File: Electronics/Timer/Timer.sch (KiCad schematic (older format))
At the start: 21 parts, among them J1 RJ12-UNSHLD, U1 74HC165, U2 MIC5504-3.3YM5

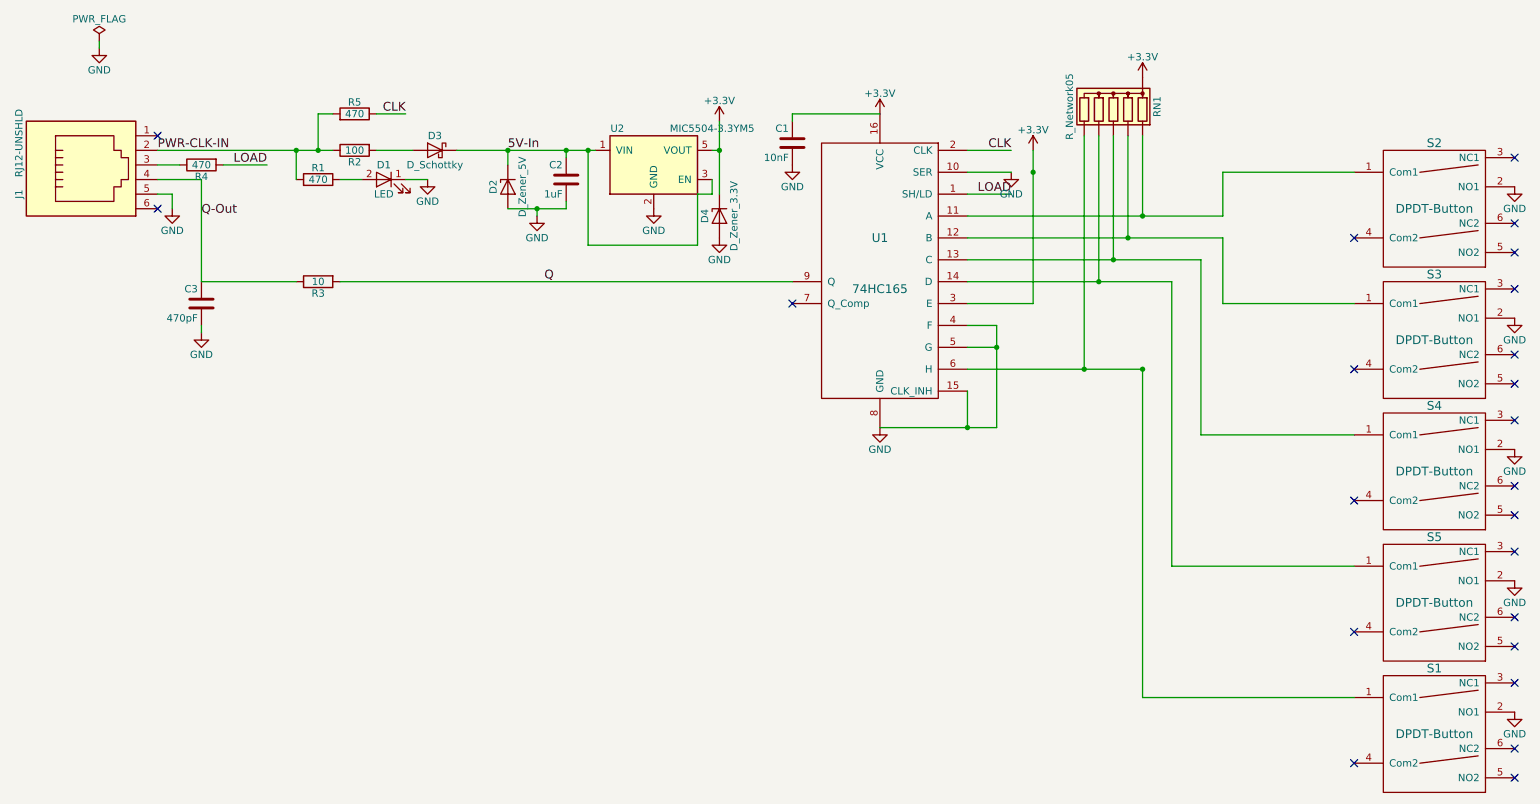
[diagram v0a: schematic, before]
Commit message: Revert "Merge branch 'master' into electronics-tweaks; overwrite 'master' hat changes"
This reverts commit 8490e2c3782f3b2eaf596155d8884dc6cd65858c, reversing
changes made to 143268d8e254d2edd056497eb53e137ee58f0f7c.
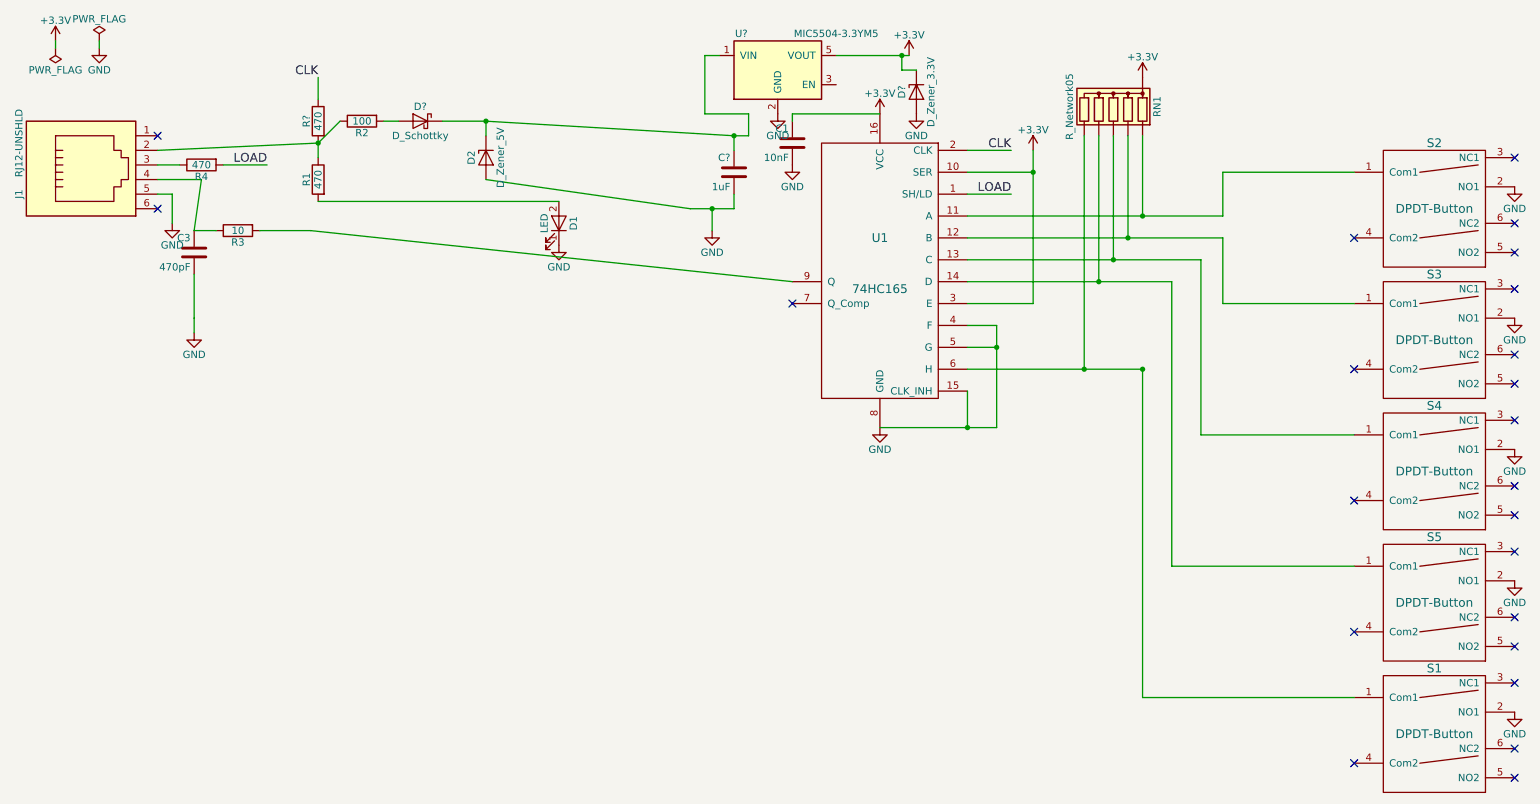
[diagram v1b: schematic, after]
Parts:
- C1: footprint Capacitors_SMD:C_0805_HandSoldering -> Capacitors_SMD:C_0603_HandSoldering
- C3: footprint Capacitors_SMD:C_1206_HandSoldering -> Capacitors_SMD:C_0603_HandSoldering
- C?: renamed from C2; footprint Capacitors_SMD:C_1206_HandSoldering -> Capacitors_SMD:C_0603_HandSoldering
- D2: footprint Diodes_SMD:D_SOD-323_HandSoldering -> Diodes_SMD:SOD-80C
- D?: renamed from D3; footprint Diodes_SMD:D_SOD-123 -> (none)
- D?: renamed from D4; footprint Diodes_SMD:D_SOD-323_HandSoldering -> Diodes_SMD:SOD-80C
- renumbered R5 to R?, U2 to U?
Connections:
- net +3V3: now also U1.10 (SER)
- net GND: no longer U1.10 (SER)
- net at R1.1: now also J1.2, R2.1, R?.2; no longer D1.2 (A)
- net 5V-In: no longer names the net of C?.1, D2.1 (K), D?.1 (K), U?.1 (VIN)
- net 5V-In: no longer U?.3 (EN)
- removed net PWR-CLK-IN: J1.2, R1.2, R2.1, R?.2
- net Q: no longer names the net of R3.2, U1.9 (Q)
- net Q-Out: no longer names the net of C3.1, J1.4, R3.1
- new net: D1.2 (A), R1.2
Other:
- moved on the sheet: C3, C?, D1, D2, D?, R2, R3, R?, U?

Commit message: Timer: Restore David's updated schematic and PCB from earlier failed merge.
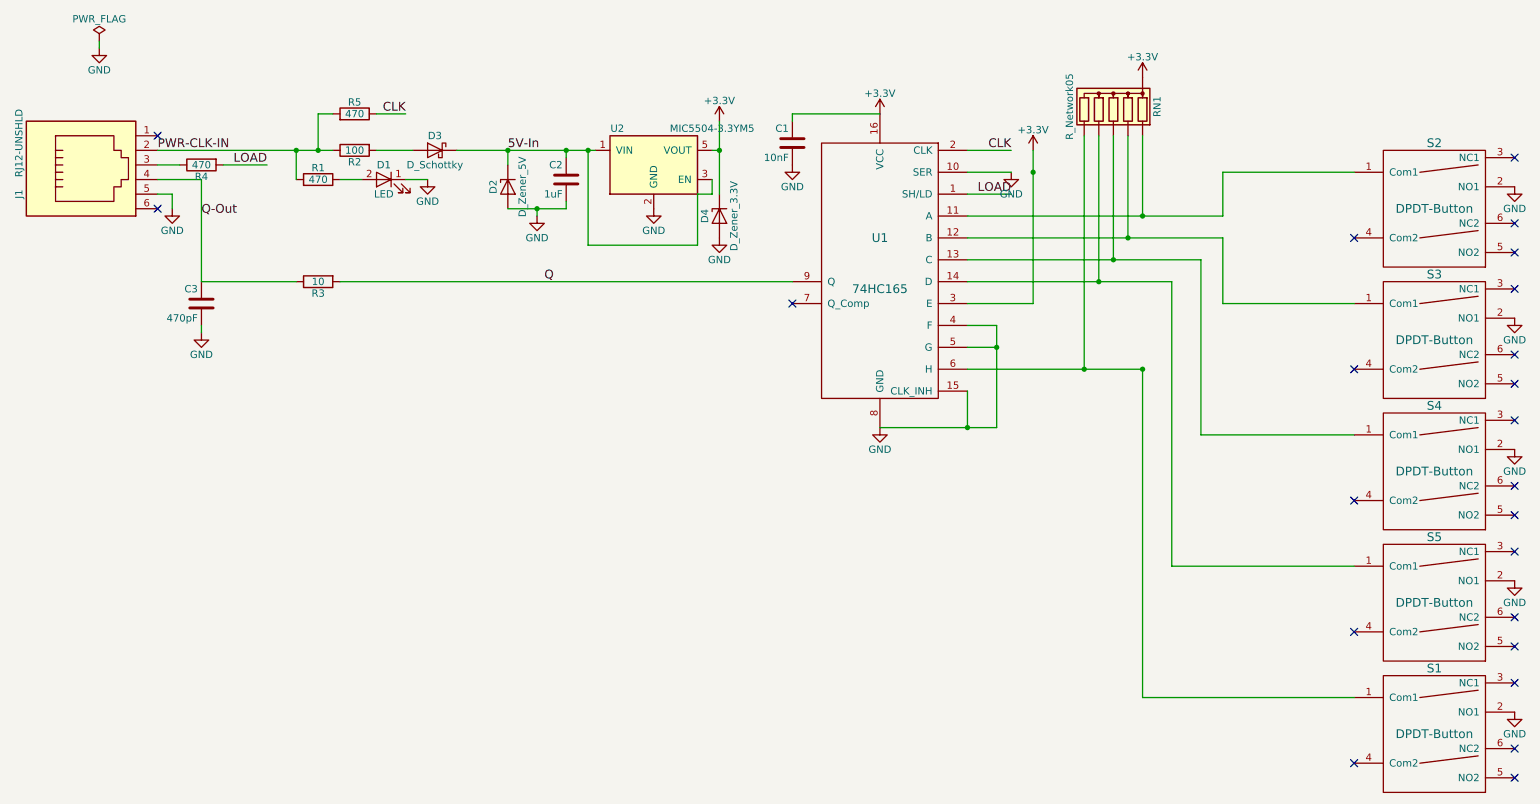
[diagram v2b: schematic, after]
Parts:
- C1: footprint Capacitors_SMD:C_0603_HandSoldering -> Capacitors_SMD:C_0805_HandSoldering
- C2: renamed from C?; footprint Capacitors_SMD:C_0603_HandSoldering -> Capacitors_SMD:C_1206_HandSoldering
- C3: footprint Capacitors_SMD:C_0603_HandSoldering -> Capacitors_SMD:C_1206_HandSoldering
- D2: footprint Diodes_SMD:SOD-80C -> Diodes_SMD:D_SOD-323_HandSoldering
- D3: renamed from D?; footprint (none) -> Diodes_SMD:D_SOD-123
- D4: renamed from D?; footprint Diodes_SMD:SOD-80C -> Diodes_SMD:D_SOD-323_HandSoldering
- gave numbers to parts that had none: 2
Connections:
- net +3V3: no longer U1.10 (SER)
- net GND: now also U1.10 (SER)
- net PWR-CLK-IN: now reaches J1.2, R2.1, R5.2
- net PWR-CLK-IN: now also R1.2; no longer R1.1
- net Q-Out: now reaches C3.1, J1.4, R3.1
- net Q: now reaches R3.2, U1.9 (Q)
- net at D1.2 (A): now also R1.1; no longer R1.2
- net 5V-In: now reaches C2.1, D2.1 (K), D3.1 (K), U2.1 (VIN)
- net 5V-In: now also U2.3 (EN)
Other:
- moved on the sheet: C2, C3, D1, D2, D3, D4, R2, R3, R5, U2
